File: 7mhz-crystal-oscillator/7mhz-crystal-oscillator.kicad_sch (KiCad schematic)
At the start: 12 parts, among them J1 Conn_Coaxial, Q1 2N3904, Y1 7MHz

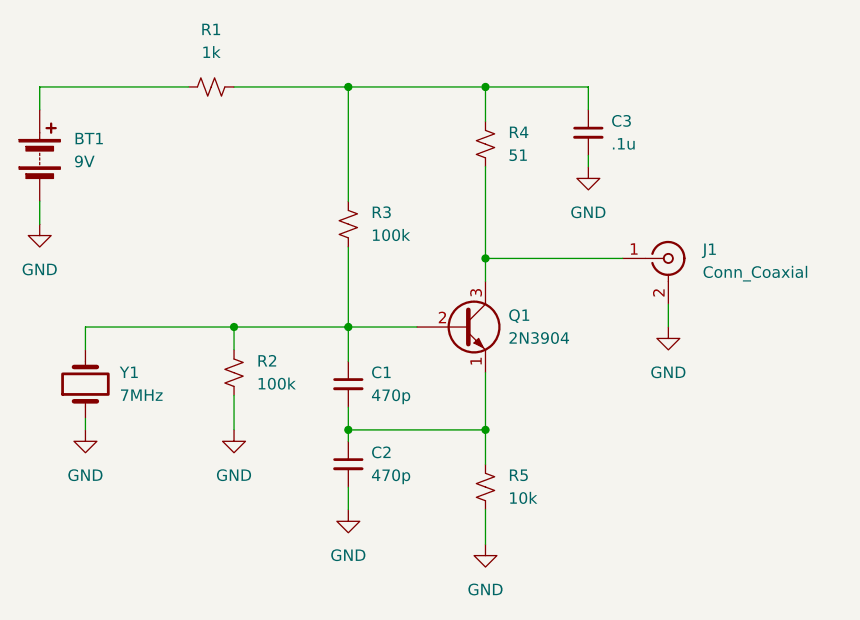
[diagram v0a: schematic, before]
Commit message: 7mhz xtal oscillator
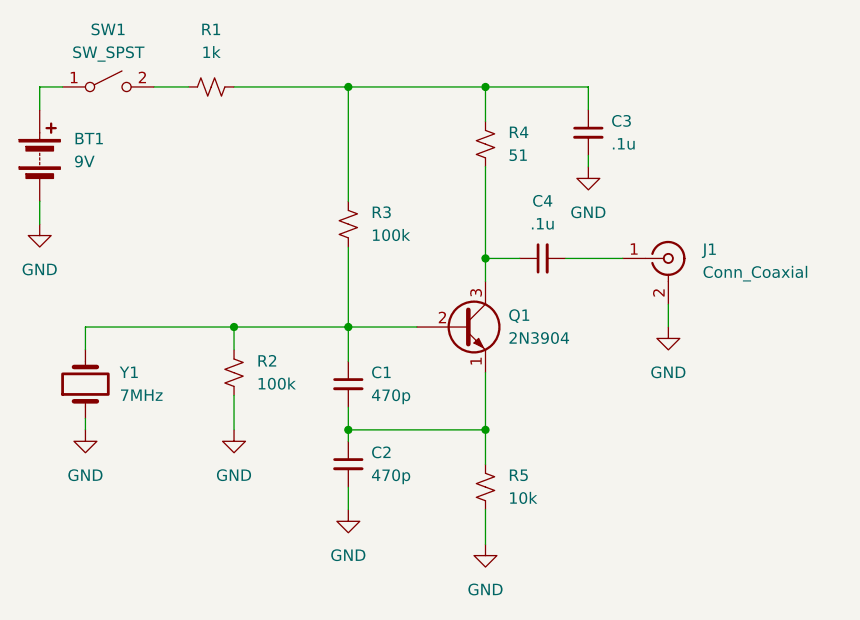
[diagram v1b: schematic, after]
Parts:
- added C4: .1u, symbol Device:C_Small
- added SW1: SW_SPST, symbol Switch:SW_SPST
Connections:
- net at Q1.3 (C), R4.2: now also C4.1; no longer J1.1 (In)
- net at R1.1: now also SW1.2 (B); no longer BT1.1 (+)
- new net: C4.2, J1.1 (In)
- new net: BT1.1 (+), SW1.1 (A)
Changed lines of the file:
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@@
     (stroke (width 0) (type default))
   )
-  (wire (pts (xy 64.77 67.31) (xy 48.26 67.31))
+  (wire (pts (xy 64.77 67.31) (xy 60.96 67.31))
     (stroke (width 0) (type default))
   )
@@
     (stroke (width 0) (type default))
   )
+  (wire (pts (xy 50.8 67.31) (xy 48.26 67.31))
+    (stroke (width 0) (type default))
+  )
   (wire (pts (xy 118.11 91.44) (xy 118.11 93.98))
     (stroke (width 0) (type default))
   )
-  (wire (pts (xy 97.79 86.36) (xy 113.03 86.36))
+  (wire (pts (xy 97.79 86.36) (xy 101.6 86.36))
     (stroke (width 0) (type default))
   )
@@
     (stroke (width 0) (type default))
   )
+  (wire (pts (xy 106.68 86.36) (xy 113.03 86.36))
+    (stroke (width 0) (type default))
+  )
   (wire (pts (xy 109.22 69.85) (xy 109.22 67.31))
     (stroke (width 0) (type default))
@@
         (path "/0b54bfea-3162-44d0-afdf-898cf06ebb22"
           (reference "#PWR01") (unit 1)
+        )
+      )
+    )
+  )
+  (symbol (lib_id "Device:C_Small") (at 104.14 86.36 90) (unit 1)
+    (in_bom yes) (on_board yes) (dnp no) (fields_autoplaced)
+    (property "Reference" "C4" (at 104.1463 80.01 90)
+      (effects (font (size 1.27 1.27)))
+    )
+    (property "Value" ".1u" (at 104.1463 82.55 90)
+      (effects (font (size 1.27 1.27)))
+    )
+    (property "Footprint" "" (at 104.14 86.36 0)
+      (effects (font (size 1.27 1.27)) hide)
+    )
+    (property "Datasheet" "~" (at 104.14 86.36 0)
+      (effects (font (size 1.27 1.27)) hide)
+    )
+    (pin "1")
+    (pin "2")
+    (instances
+      (project "7mhz-crystal-oscillator"
+        (path "/0b54bfea-3162-44d0-afdf-898cf06ebb22"
+          (reference "C4") (unit 1)
         )
       )
@@
         )
       )
+    )
+  )
+  (symbol (lib_id "Switch:SW_SPST") (at 55.88 67.31 0) (unit 1)
+    (in_bom yes) (on_board yes) (dnp no) (fields_autoplaced)
+    (property "Reference" "SW1" (at 55.88 60.96 0)
+      (effects (font (size 1.27 1.27)))
+    )
+    (property "Value" "SW_SPST" (at 55.88 63.5 0)
+      (effects (font (size 1.27 1.27)))
+    )
+    (property "Footprint" "" (at 55.88 67.31 0)
+      (effects (font (size 1.27 1.27)) hide)
+    )
+    (property "Datasheet" "~" (at 55.88 67.31 0)
+      (effects (font (size 1.27 1.27)) hide)
+    )
+    (pin "2")
+    (pin "1")
+    (instances
+      (project "7mhz-crystal-oscillator"
+        (path "/0b54bfea-3162-44d0-afdf-898cf06ebb22"
+          (reference "SW1") (unit 1)
+        )
+      )
